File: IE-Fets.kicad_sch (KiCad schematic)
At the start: 11 parts

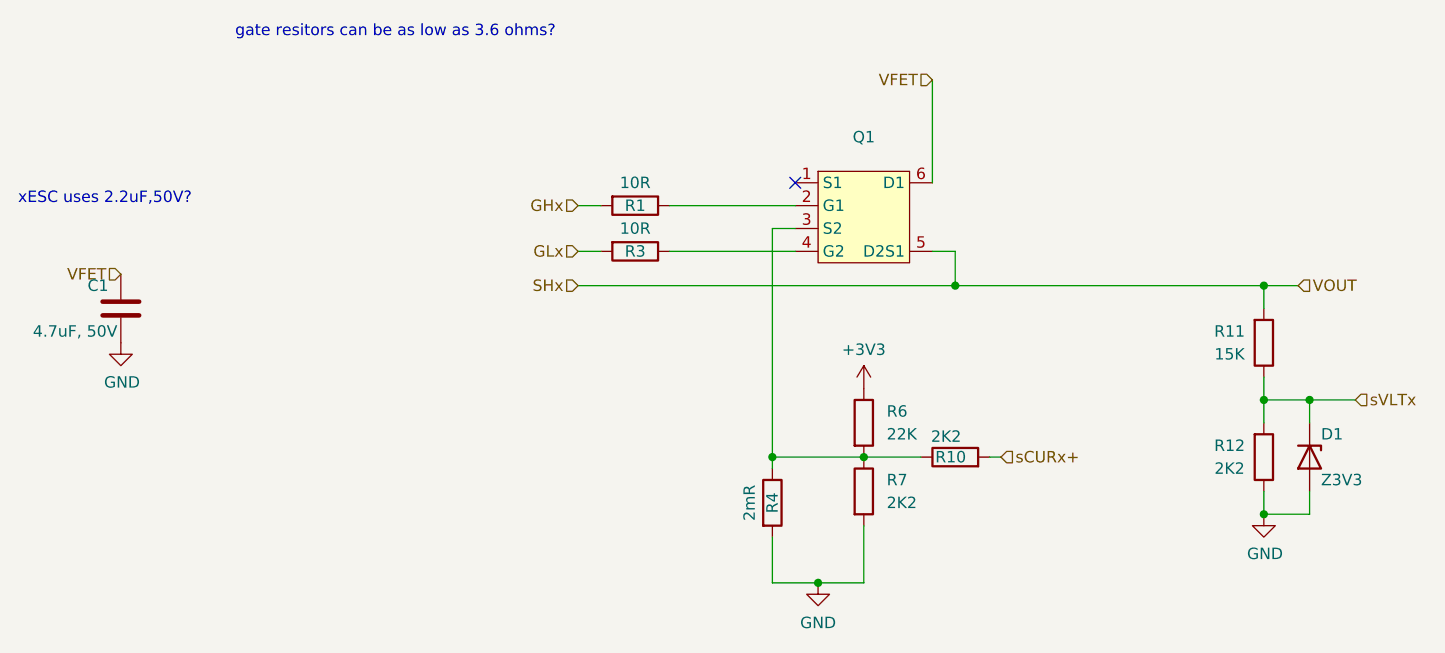
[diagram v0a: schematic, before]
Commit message: schematic fix before re-org
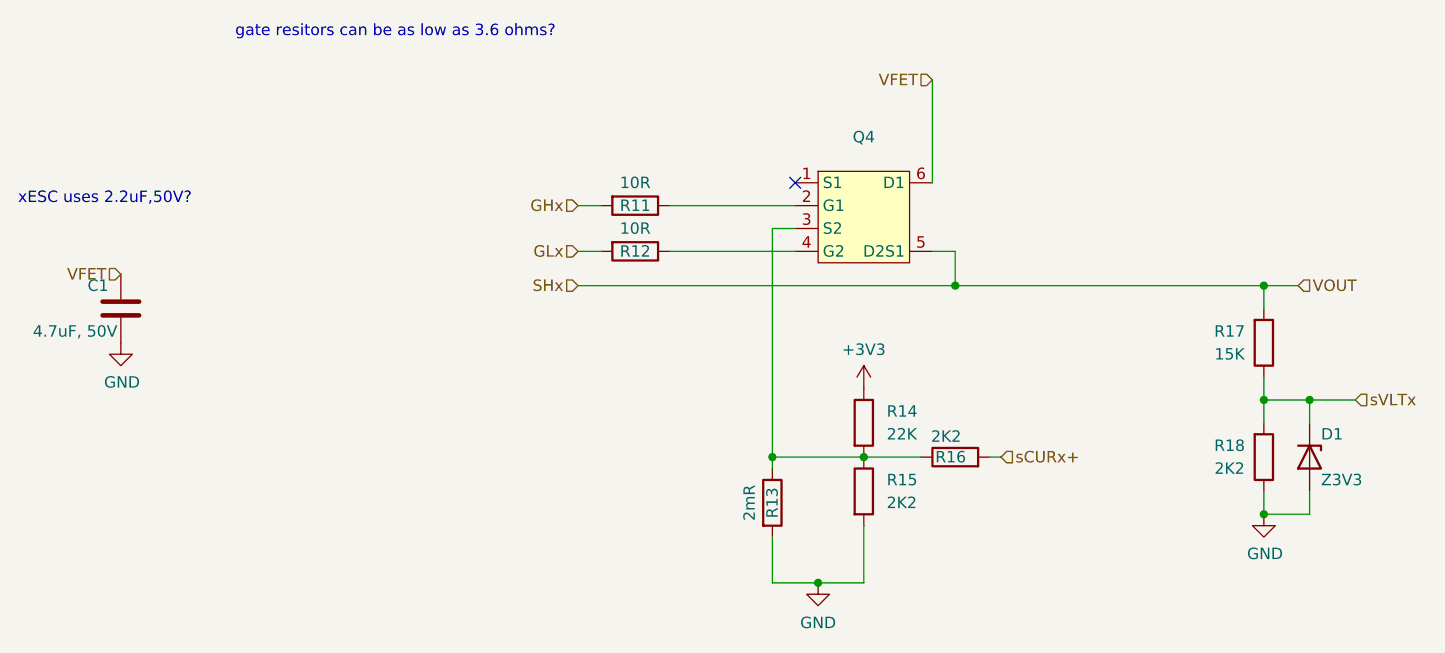
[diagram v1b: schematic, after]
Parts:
- renumbered Q1 to Q4, R1 to R11, R3 to R12, R4 to R13, R6 to R14, R7 to R15, R10 to R16, R11 to R17, R12 to R18

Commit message: push before schematic cleanup
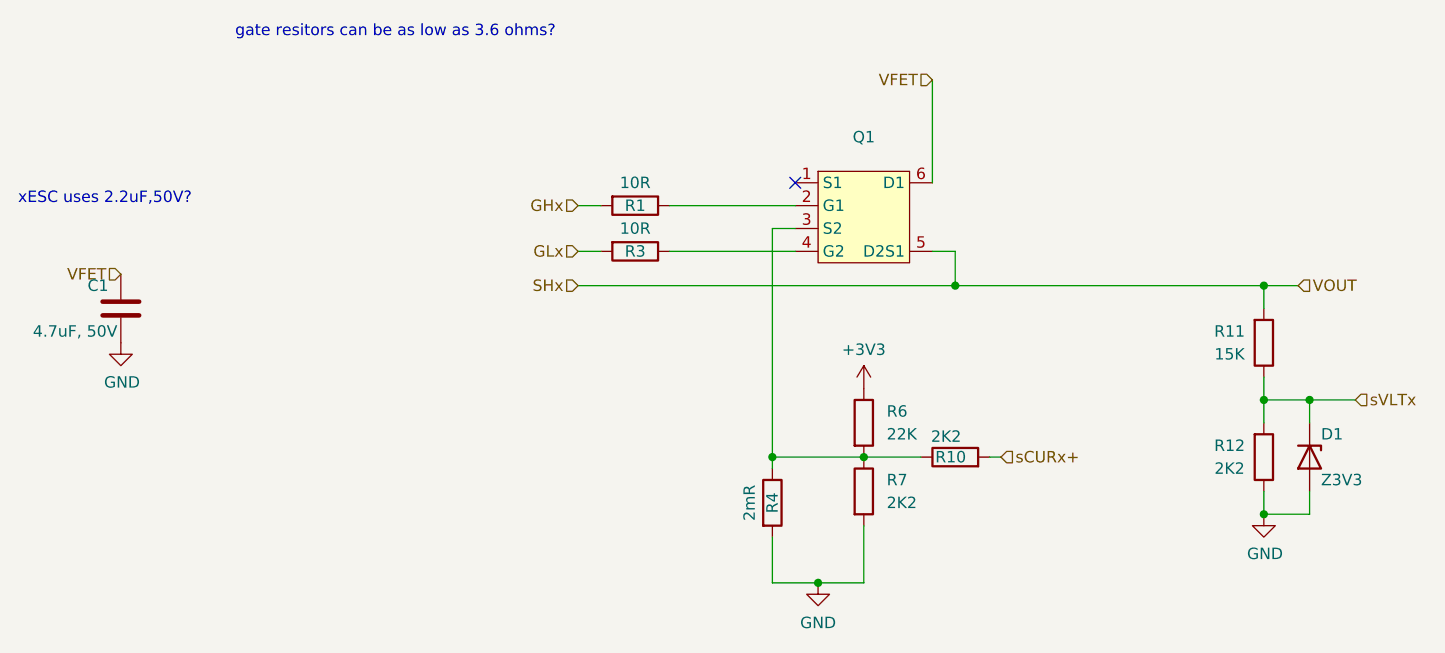
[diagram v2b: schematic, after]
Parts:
- renumbered Q4 to Q1, R11 to R1, R16 to R10, R17 to R11, R18 to R12, R12 to R3, R13 to R4, R14 to R6, R15 to R7
